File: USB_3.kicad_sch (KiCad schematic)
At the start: 0 parts

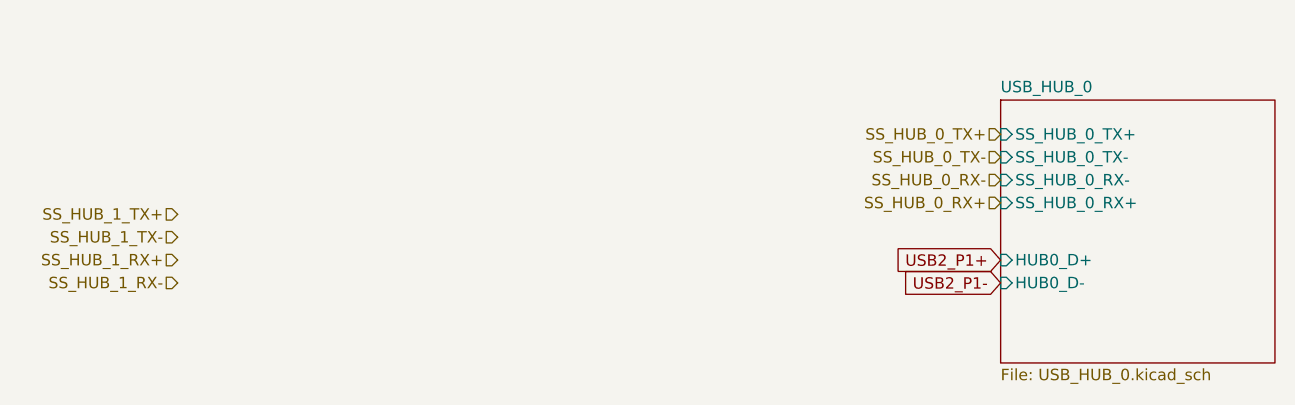
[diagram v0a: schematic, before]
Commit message: .
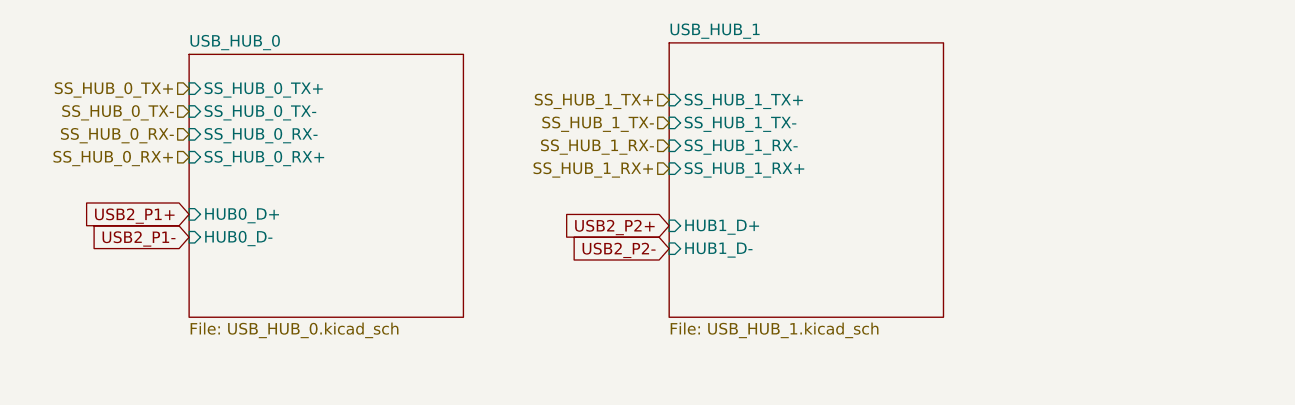
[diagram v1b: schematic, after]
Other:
- added sheet USB_HUB_1 (USB_HUB_1.kicad_sch)
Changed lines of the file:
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@@
 	(generator_version "9.0")
 	(paper "A4")
-	(global_label "USB2_P1+"
-		(shape input)
-		(at 147.32 48.26 180)
+	(global_label "USB2_P2-"
+		(shape input)
+		(at 110.49 46.99 180)
 		(fields_autoplaced yes)
 		(effects
@@
 		)
 		(property "Intersheetrefs" "${INTERSHEET_REFS}"
-			(at 134.2958 48.26 0)
+			(at 97.4658 46.99 0)
 			(effects
 				(font
@@
 		)
 	)
-	(global_label "USB2_P1-"
-		(shape input)
-		(at 147.32 50.8 180)
+	(global_label "USB2_P1+"
+		(shape input)
+		(at 57.15 43.18 180)
 		(fields_autoplaced yes)
 		(effects
@@
 		)
 		(property "Intersheetrefs" "${INTERSHEET_REFS}"
-			(at 134.2958 50.8 0)
+			(at 44.1258 43.18 0)
 			(effects
 				(font
@@
 		)
 	)
+	(global_label "USB2_P2+"
+		(shape input)
+		(at 110.49 44.45 180)
+		(fields_autoplaced yes)
+		(effects
+			(font
+				(size 1.27 1.27)
+				(color 255 255 255 1)
+			)
+			(justify right)
+		)
+		(property "Intersheetrefs" "${INTERSHEET_REFS}"
+			(at 97.4658 44.45 0)
+			(effects
+				(font
+					(size 1.27 1.27)
+				)
+				(justify right)
+				(hide yes)
+			)
+		)
+	)
+	(global_label "USB2_P1-"
+		(shape input)
+		(at 57.15 45.72 180)
+		(fields_autoplaced yes)
+		(effects
+			(font
+				(size 1.27 1.27)
+				(color 255 255 255 1)
+			)
+			(justify right)
+		)
+		(property "Intersheetrefs" "${INTERSHEET_REFS}"
+			(at 44.1258 45.72 0)
+			(effects
+				(font
+					(size 1.27 1.27)
+				)
+				(justify right)
+				(hide yes)
+			)
+		)
+	)
+	(hierarchical_label "SS_HUB_0_RX+"
+		(shape input)
+		(at 57.15 36.83 180)
+		(effects
+			(font
+				(size 1.27 1.27)
+			)
+			(justify right)
+		)
+	)
+	(hierarchical_label "SS_HUB_1_RX-"
+		(shape input)
+		(at 110.49 35.56 180)
+		(effects
+			(font
+				(size 1.27 1.27)
+			)
+			(justify right)
+		)
+	)
+	(hierarchical_label "SS_HUB_1_RX+"
+		(shape input)
+		(at 110.49 38.1 180)
+		(effects
+			(font
+				(size 1.27 1.27)
+			)
+			(justify right)
+		)
+	)
+	(hierarchical_label "SS_HUB_1_TX+"
+		(shape input)
+		(at 110.49 30.48 180)
+		(effects
+			(font
+				(size 1.27 1.27)
+			)
+			(justify right)
+		)
+	)
+	(hierarchical_label "SS_HUB_0_TX-"
+		(shape input)
+		(at 57.15 31.75 180)
+		(effects
+			(font
+				(size 1.27 1.27)
+			)
+			(justify right)
+		)
+	)
+	(hierarchical_label "SS_HUB_0_RX-"
+		(shape input)
+		(at 57.15 34.29 180)
+		(effects
+			(font
+				(size 1.27 1.27)
+			)
+			(justify right)
+		)
+	)
+	(hierarchical_label "SS_HUB_0_TX+"
+		(shape input)
+		(at 57.15 29.21 180)
+		(effects
+			(font
+				(size 1.27 1.27)
+			)
+			(justify right)
+		)
+	)
 	(hierarchical_label "SS_HUB_1_TX-"
 		(shape input)
-		(at 55.88 45.72 180)
-		(effects
-			(font
-				(size 1.27 1.27)
-			)
-			(justify right)
-		)
-	)
-	(hierarchical_label "SS_HUB_0_RX+"
-		(shape input)
-		(at 147.32 41.91 180)
-		(effects
-			(font
-				(size 1.27 1.27)
-			)
-			(justify right)
-		)
-	)
-	(hierarchical_label "SS_HUB_1_RX-"
-		(shape input)
-		(at 55.88 50.8 180)
-		(effects
-			(font
-				(size 1.27 1.27)
-			)
-			(justify right)
-		)
-	)
-	(hierarchical_label "SS_HUB_1_TX+"
-		(shape input)
-		(at 55.88 43.18 180)
-		(effects
-			(font
-				(size 1.27 1.27)
-			)
-			(justify right)
-		)
-	)
-	(hierarchical_label "SS_HUB_0_TX-"
-		(shape input)
-		(at 147.32 36.83 180)
-		(effects
-			(font
-				(size 1.27 1.27)
-			)
-			(justify right)
-		)
-	)
-	(hierarchical_label "SS_HUB_0_RX-"
-		(shape input)
-		(at 147.32 39.37 180)
-		(effects
-			(font
-				(size 1.27 1.27)
-			)
-			(justify right)
-		)
-	)
-	(hierarchical_label "SS_HUB_0_TX+"
-		(shape input)
-		(at 147.32 34.29 180)
-		(effects
-			(font
-				(size 1.27 1.27)
-			)
-			(justify right)
-		)
-	)
-	(hierarchical_label "SS_HUB_1_RX+"
-		(shape input)
-		(at 55.88 48.26 180)
+		(at 110.49 33.02 180)
 		(effects
 			(font
@@
 	)
 	(sheet
-		(at 147.32 30.48)
+		(at 57.15 25.4)
 		(size 30.48 29.21)
 		(exclude_from_sim no)
@@
 		)
 		(property "Sheetname" "USB_HUB_0"
-			(at 147.32 29.7684 0)
+			(at 57.15 24.6884 0)
 			(effects
 				(font
@@
 		)
 		(property "Sheetfile" "USB_HUB_0.kicad_sch"
-			(at 147.32 60.2746 0)
+			(at 57.15 55.1946 0)
 			(effects
 				(font
@@
 		)
 		(pin "SS_HUB_0_TX+" input
-			(at 147.32 34.29 180)
+			(at 57.15 29.21 180)
 			(effects
 				(font
@@
 		)
 		(pin "SS_HUB_0_RX-" input
-			(at 147.32 39.37 180)
+			(at 57.15 34.29 180)
 			(effects
 				(font
@@
 		)
 		(pin "SS_HUB_0_RX+" input
-			(at 147.32 41.91 180)
+			(at 57.15 36.83 180)
 			(effects
 				(font
@@
 		)
 		(pin "SS_HUB_0_TX-" input
-			(at 147.32 36.83 180)
+			(at 57.15 31.75 180)
 			(effects
 				(font
@@
 		)
 		(pin "HUB0_D+" input
-			(at 147.32 48.26 180)
+			(at 57.15 43.18 180)
 			(effects
 				(font
@@
 		)
 		(pin "HUB0_D-" input
-			(at 147.32 50.8 180)
+			(at 57.15 45.72 180)
 			(effects
 				(font
@@
 				)
 			)
+		)
+	)
+	(sheet
+		(at 110.49 24.13)
+		(size 30.48 30.48)
+		(exclude_from_sim no)
+		(in_bom yes)
+		(on_board yes)
+		(dnp no)
+		(fields_autoplaced yes)
+		(stroke
+			(width 0.1524)
+			(type solid)
+		)
+		(fill
+			(color 0 0 0 0.0000)
+		)
+		(property "Sheetname" "USB_HUB_1"
+			(at 110.49 23.4184 0)
+			(effects
+				(font
+					(size 1.27 1.27)
+				)
+				(justify left bottom)
+			)
+		)
+		(property "Sheetfile" "USB_HUB_1.kicad_sch"
+			(at 110.49 55.1946 0)
+			(effects
+				(font
+					(size 1.27 1.27)
+				)
+				(justify left top)
+			)
+		)
+		(pin "SS_HUB_1_TX-" input
+			(at 110.49 33.02 180)
+			(effects
+				(font
+					(size 1.27 1.27)
+				)
+				(justify left)
+			)
+		)
+		(pin "SS_HUB_1_TX+" input
+			(at 110.49 30.48 180)
+			(effects
+				(font
+					(size 1.27 1.27)
+				)
+				(justify left)
+			)
+		)
+		(pin "HUB1_D+" input
+			(at 110.49 44.45 180)
+			(effects
+				(font
+					(size 1.27 1.27)
+				)
+				(justify left)
+			)
+		)
+		(pin "SS_HUB_1_RX+" input
+			(at 110.49 38.1 180)
+			(effects
+				(font
+					(size 1.27 1.27)
+				)
+				(justify left)
+			)
+		)
+		(pin "HUB1_D-" input
+			(at 110.49 46.99 180)
+			(effects
+				(font
+					(size 1.27 1.27)
+				)
+				(justify left)
+			)
+		)
+		(pin "SS_HUB_1_RX-" input
+			(at 110.49 35.56 180)
+			(effects
+				(font
+					(size 1.27 1.27)
+				)
+				(justify left)
+			)
+		)
+		(instances
+			(project "MiniLatte"
+				(path "/ffe475c5-d6e9-41b5-8ca1-322659dd88d8/9db433ce-ea3f-4d40-ac5c-6665012436f8"
+					(page "11")
+				)
+			)

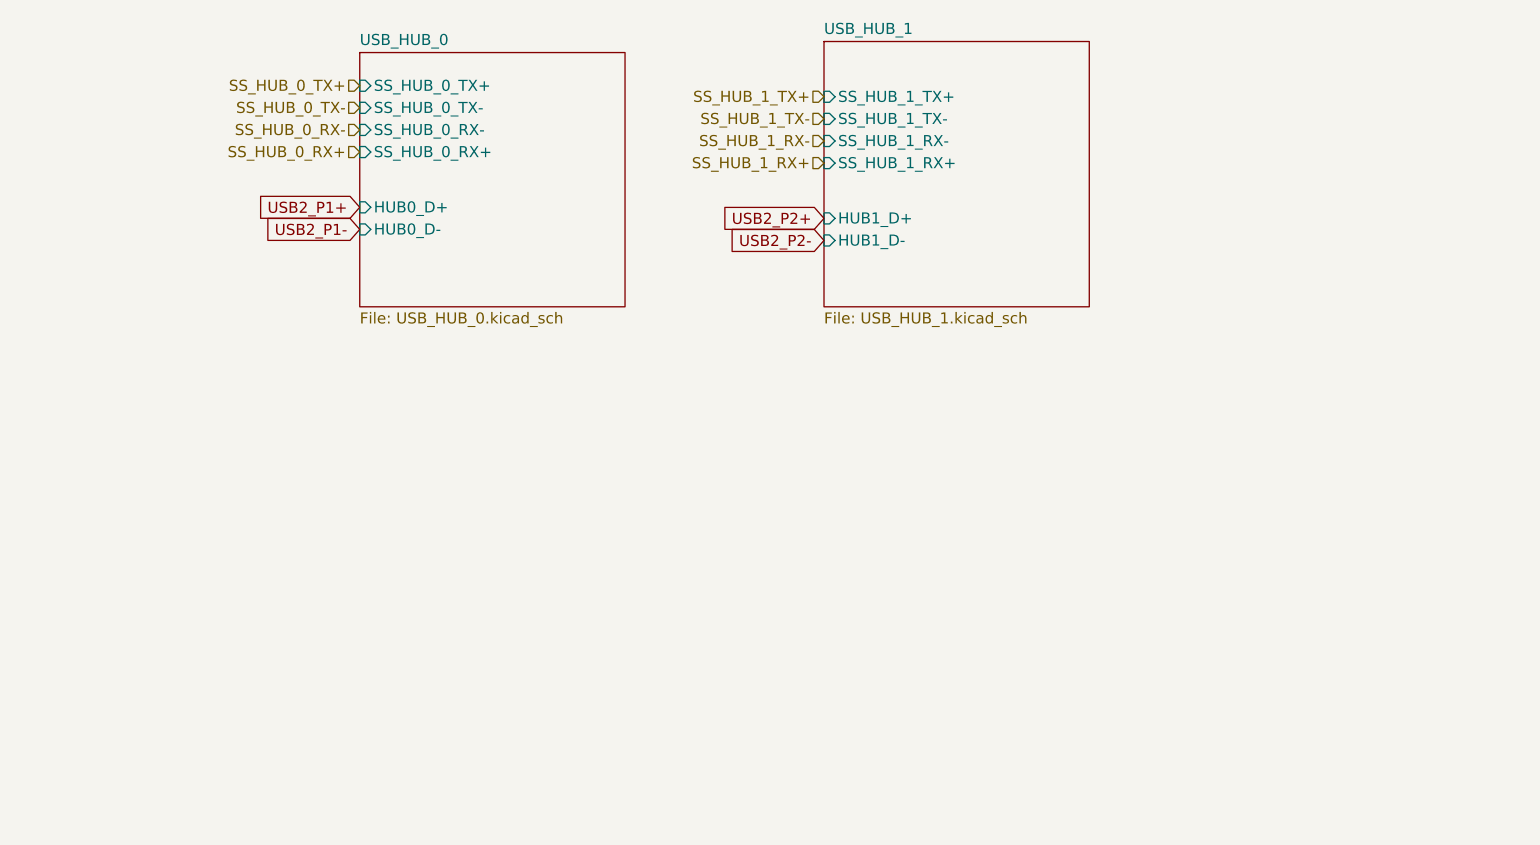
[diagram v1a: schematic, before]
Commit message: .
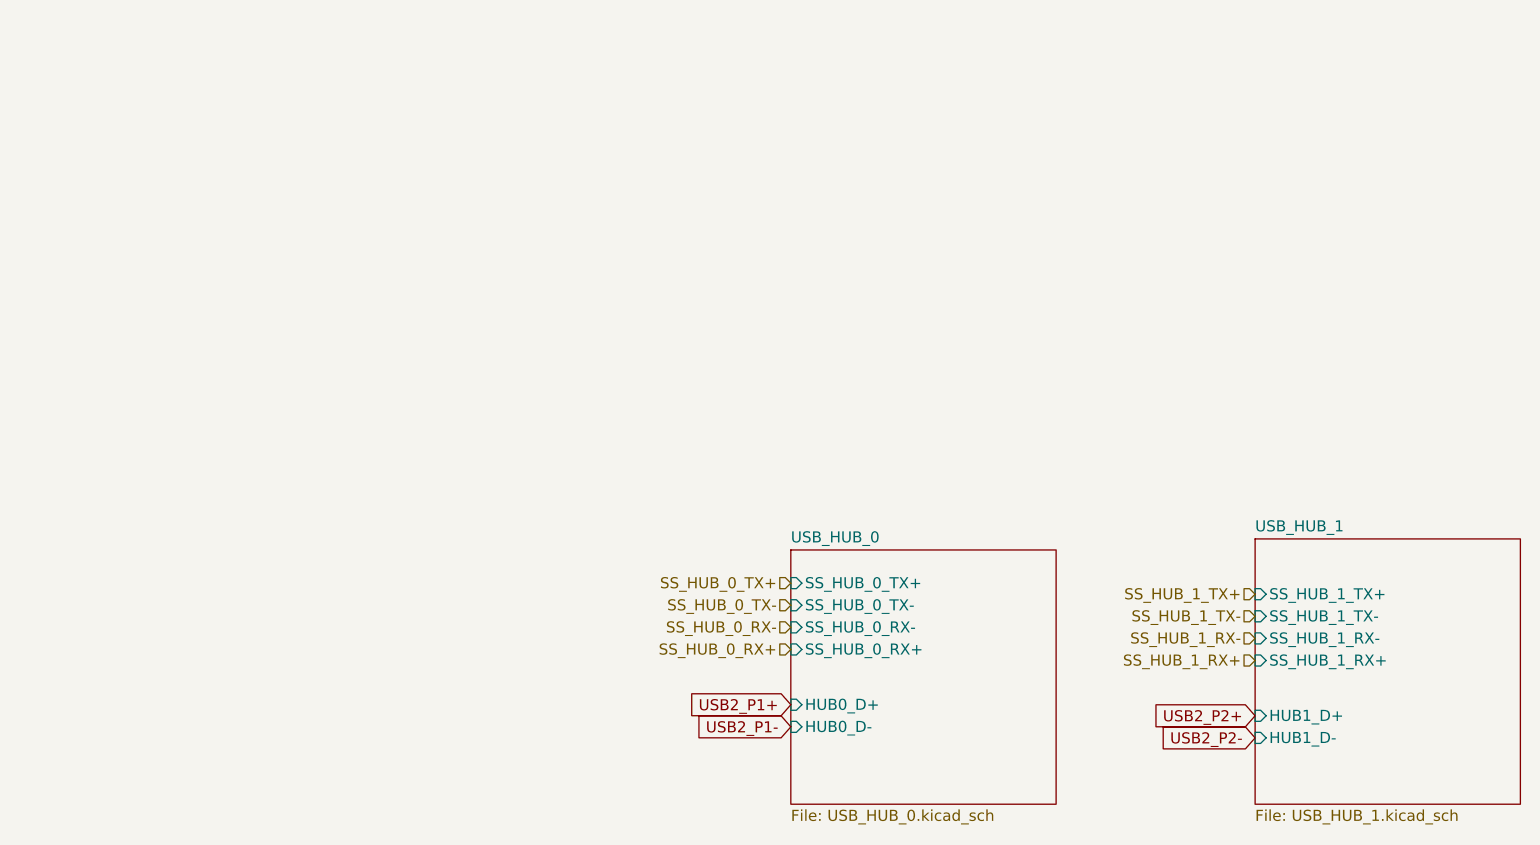
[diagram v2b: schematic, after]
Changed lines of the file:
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@@
 	(global_label "USB2_P2-"
 		(shape input)
-		(at 110.49 46.99 180)
+		(at 160.02 104.14 180)
 		(fields_autoplaced yes)
 		(effects
@@
 		)
 		(property "Intersheetrefs" "${INTERSHEET_REFS}"
-			(at 97.4658 46.99 0)
+			(at 146.9958 104.14 0)
 			(effects
 				(font
@@
 	(global_label "USB2_P1+"
 		(shape input)
-		(at 57.15 43.18 180)
+		(at 106.68 100.33 180)
 		(fields_autoplaced yes)
 		(effects
@@
 		)
 		(property "Intersheetrefs" "${INTERSHEET_REFS}"
-			(at 44.1258 43.18 0)
+			(at 93.6558 100.33 0)
 			(effects
 				(font
@@
 	(global_label "USB2_P2+"
 		(shape input)
-		(at 110.49 44.45 180)
+		(at 160.02 101.6 180)
 		(fields_autoplaced yes)
 		(effects
@@
 		)
 		(property "Intersheetrefs" "${INTERSHEET_REFS}"
-			(at 97.4658 44.45 0)
+			(at 146.9958 101.6 0)
 			(effects
 				(font
@@
 	(global_label "USB2_P1-"
 		(shape input)
-		(at 57.15 45.72 180)
+		(at 106.68 102.87 180)
 		(fields_autoplaced yes)
 		(effects
@@
 		)
 		(property "Intersheetrefs" "${INTERSHEET_REFS}"
-			(at 44.1258 45.72 0)
+			(at 93.6558 102.87 0)
 			(effects
 				(font
@@
 	(hierarchical_label "SS_HUB_0_RX+"
 		(shape input)
-		(at 57.15 36.83 180)
+		(at 106.68 93.98 180)
 		(effects
 			(font
@@
 	(hierarchical_label "SS_HUB_1_RX-"
 		(shape input)
-		(at 110.49 35.56 180)
+		(at 160.02 92.71 180)
 		(effects
 			(font
@@
 	(hierarchical_label "SS_HUB_1_RX+"
 		(shape input)
-		(at 110.49 38.1 180)
+		(at 160.02 95.25 180)
 		(effects
 			(font
@@
 	(hierarchical_label "SS_HUB_1_TX+"
 		(shape input)
-		(at 110.49 30.48 180)
+		(at 160.02 87.63 180)
 		(effects
 			(font
@@
 	(hierarchical_label "SS_HUB_0_TX-"
 		(shape input)
-		(at 57.15 31.75 180)
+		(at 106.68 88.9 180)
 		(effects
 			(font
@@
 	(hierarchical_label "SS_HUB_0_RX-"
 		(shape input)
-		(at 57.15 34.29 180)
+		(at 106.68 91.44 180)
 		(effects
 			(font
@@
 	(hierarchical_label "SS_HUB_0_TX+"
 		(shape input)
-		(at 57.15 29.21 180)
+		(at 106.68 86.36 180)
 		(effects
 			(font
@@
 	(hierarchical_label "SS_HUB_1_TX-"
 		(shape input)
-		(at 110.49 33.02 180)
+		(at 160.02 90.17 180)
 		(effects
 			(font
@@
 	)
 	(sheet
-		(at 57.15 25.4)
+		(at 106.68 82.55)
 		(size 30.48 29.21)
 		(exclude_from_sim no)
@@
 		)
 		(property "Sheetname" "USB_HUB_0"
-			(at 57.15 24.6884 0)
+			(at 106.68 81.8384 0)
 			(effects
 				(font
@@
 		)
 		(property "Sheetfile" "USB_HUB_0.kicad_sch"
-			(at 57.15 55.1946 0)
+			(at 106.68 112.3446 0)
 			(effects
 				(font
@@
 		)
 		(pin "SS_HUB_0_TX+" input
-			(at 57.15 29.21 180)
+			(at 106.68 86.36 180)
 			(effects
 				(font
@@
 		)
 		(pin "SS_HUB_0_RX-" input
-			(at 57.15 34.29 180)
+			(at 106.68 91.44 180)
 			(effects
 				(font
@@
 		)
 		(pin "SS_HUB_0_RX+" input
-			(at 57.15 36.83 180)
+			(at 106.68 93.98 180)
 			(effects
 				(font
@@
 		)
 		(pin "SS_HUB_0_TX-" input
-			(at 57.15 31.75 180)
+			(at 106.68 88.9 180)
 			(effects
 				(font
@@
 		)
 		(pin "HUB0_D+" input
-			(at 57.15 43.18 180)
+			(at 106.68 100.33 180)
 			(effects
 				(font
@@
 		)
 		(pin "HUB0_D-" input
-			(at 57.15 45.72 180)
+			(at 106.68 102.87 180)
 			(effects
 				(font
@@
 	)
 	(sheet
-		(at 110.49 24.13)
+		(at 160.02 81.28)
 		(size 30.48 30.48)
 		(exclude_from_sim no)
@@
 		)
 		(property "Sheetname" "USB_HUB_1"
-			(at 110.49 23.4184 0)
+			(at 160.02 80.5684 0)
 			(effects
 				(font
@@
 		)
 		(property "Sheetfile" "USB_HUB_1.kicad_sch"
-			(at 110.49 55.1946 0)
+			(at 160.02 112.3446 0)
 			(effects
 				(font
@@
 		)
 		(pin "SS_HUB_1_TX-" input
-			(at 110.49 33.02 180)
+			(at 160.02 90.17 180)
 			(effects
 				(font
@@
 		)
 		(pin "SS_HUB_1_TX+" input
-			(at 110.49 30.48 180)
+			(at 160.02 87.63 180)
 			(effects
 				(font
@@
 		)
 		(pin "HUB1_D+" input
-			(at 110.49 44.45 180)
+			(at 160.02 101.6 180)
 			(effects
 				(font
@@
 		)
 		(pin "SS_HUB_1_RX+" input
-			(at 110.49 38.1 180)
+			(at 160.02 95.25 180)
 			(effects
 				(font
@@
 		)
 		(pin "HUB1_D-" input
-			(at 110.49 46.99 180)
+			(at 160.02 104.14 180)
 			(effects
 				(font
@@
 		)
 		(pin "SS_HUB_1_RX-" input
-			(at 110.49 35.56 180)
-			(effects
-				(font
+			(at 160.02 92.71 180)
+			(effects
+				(font

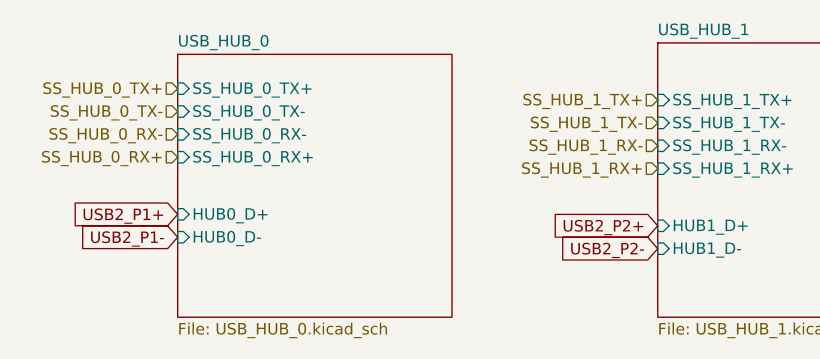
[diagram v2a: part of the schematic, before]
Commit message: .
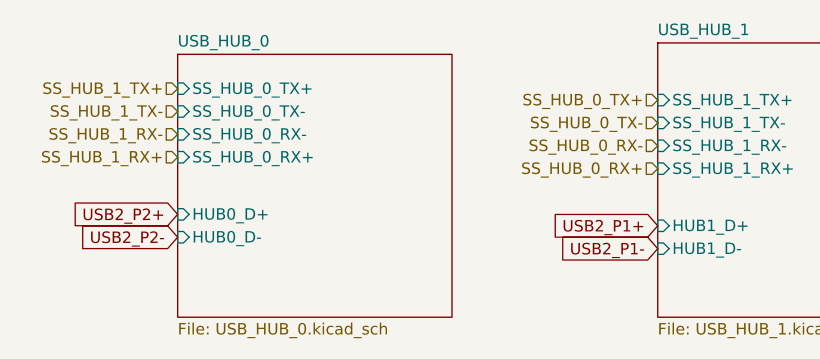
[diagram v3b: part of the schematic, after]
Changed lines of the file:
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@@
 	(global_label "USB2_P2-"
 		(shape input)
-		(at 160.02 104.14 180)
+		(at 106.68 102.87 180)
 		(fields_autoplaced yes)
 		(effects
@@
 		)
 		(property "Intersheetrefs" "${INTERSHEET_REFS}"
-			(at 146.9958 104.14 0)
+			(at 93.6558 102.87 0)
 			(effects
 				(font
@@
 		)
 	)
-	(global_label "USB2_P1+"
+	(global_label "USB2_P2+"
 		(shape input)
 		(at 106.68 100.33 180)
@@
 		)
 	)
-	(global_label "USB2_P2+"
+	(global_label "USB2_P1+"
 		(shape input)
 		(at 160.02 101.6 180)
@@
 	(global_label "USB2_P1-"
 		(shape input)
-		(at 106.68 102.87 180)
+		(at 160.02 104.14 180)
 		(fields_autoplaced yes)
 		(effects
@@
 		)
 		(property "Intersheetrefs" "${INTERSHEET_REFS}"
-			(at 93.6558 102.87 0)
+			(at 146.9958 104.14 0)
 			(effects
 				(font
@@
 		)
 	)
-	(hierarchical_label "SS_HUB_0_RX+"
+	(hierarchical_label "SS_HUB_1_RX-"
 		(shape input)
-		(at 106.68 93.98 180)
+		(at 106.68 91.44 180)
 		(effects
 			(font
@@
 		)
 	)
-	(hierarchical_label "SS_HUB_1_RX-"
+	(hierarchical_label "SS_HUB_1_TX+"
+		(shape input)
+		(at 106.68 86.36 180)
+		(effects
+			(font
+				(size 1.27 1.27)
+			)
+			(justify right)
+		)
+	)
+	(hierarchical_label "SS_HUB_0_TX+"
+		(shape input)
+		(at 160.02 87.63 180)
+		(effects
+			(font
+				(size 1.27 1.27)
+			)
+			(justify right)
+		)
+	)
+	(hierarchical_label "SS_HUB_0_RX+"
+		(shape input)
+		(at 160.02 95.25 180)
+		(effects
+			(font
+				(size 1.27 1.27)
+			)
+			(justify right)
+		)
+	)
+	(hierarchical_label "SS_HUB_1_TX-"
+		(shape input)
+		(at 106.68 88.9 180)
+		(effects
+			(font
+				(size 1.27 1.27)
+			)
+			(justify right)
+		)
+	)
+	(hierarchical_label "SS_HUB_0_TX-"
+		(shape input)
+		(at 160.02 90.17 180)
+		(effects
+			(font
+				(size 1.27 1.27)
+			)
+			(justify right)
+		)
+	)
+	(hierarchical_label "SS_HUB_0_RX-"
 		(shape input)
 		(at 160.02 92.71 180)
@@
 	(hierarchical_label "SS_HUB_1_RX+"
 		(shape input)
-		(at 160.02 95.25 180)
+		(at 106.68 93.98 180)
 		(effects
 			(font
-				(size 1.27 1.27)
-			)
-			(justify right)
-		)
-	)
-	(hierarchical_label "SS_HUB_1_TX+"
-		(shape input)
-		(at 160.02 87.63 180)
-		(effects
-			(font
-				(size 1.27 1.27)
-			)
-			(justify right)
-		)
-	)
-	(hierarchical_label "SS_HUB_0_TX-"
-		(shape input)
-		(at 106.68 88.9 180)
-		(effects
-			(font
-				(size 1.27 1.27)
-			)
-			(justify right)
-		)
-	)
-	(hierarchical_label "SS_HUB_0_RX-"
-		(shape input)
-		(at 106.68 91.44 180)
-		(effects
-			(font
-				(size 1.27 1.27)
-			)
-			(justify right)
-		)
-	)
-	(hierarchical_label "SS_HUB_0_TX+"
-		(shape input)
-		(at 106.68 86.36 180)
-		(effects
-			(font
-				(size 1.27 1.27)
-			)
-			(justify right)
-		)
-	)
-	(hierarchical_label "SS_HUB_1_TX-"
-		(shape input)
-		(at 160.02 90.17 180)
-		(effects
-			(font
